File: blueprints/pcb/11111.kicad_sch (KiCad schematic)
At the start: 64 parts, among them J1 AudioJack4, SW1 SW_Push, SW10 SW_Push, SW11 SW_Push, SW12 SW_Push, SW13 SW_Push, SW14 SW_Push, SW15 SW_Push, SW16 SW_Push, SW17 SW_Push, SW18 SW_Push, SW19 SW_Push, SW2 SW_Push, SW20 SW_Push, SW21 SW_Push, SW22 SW_Push, SW23 SW_Push, SW24 SW_Push, SW25 SW_Push, SW26 SW_Push, SW27 SW_Push, SW28 SW_Push, SW29 SW_Push, SW3 SW_Push, SW30 SW_Push, SW31 SW_Push, SW4 SW_Push, SW5 SW_Push, SW6 SW_Push, SW7 SW_Push, SW8 SW_Push, SW9 SW_Push

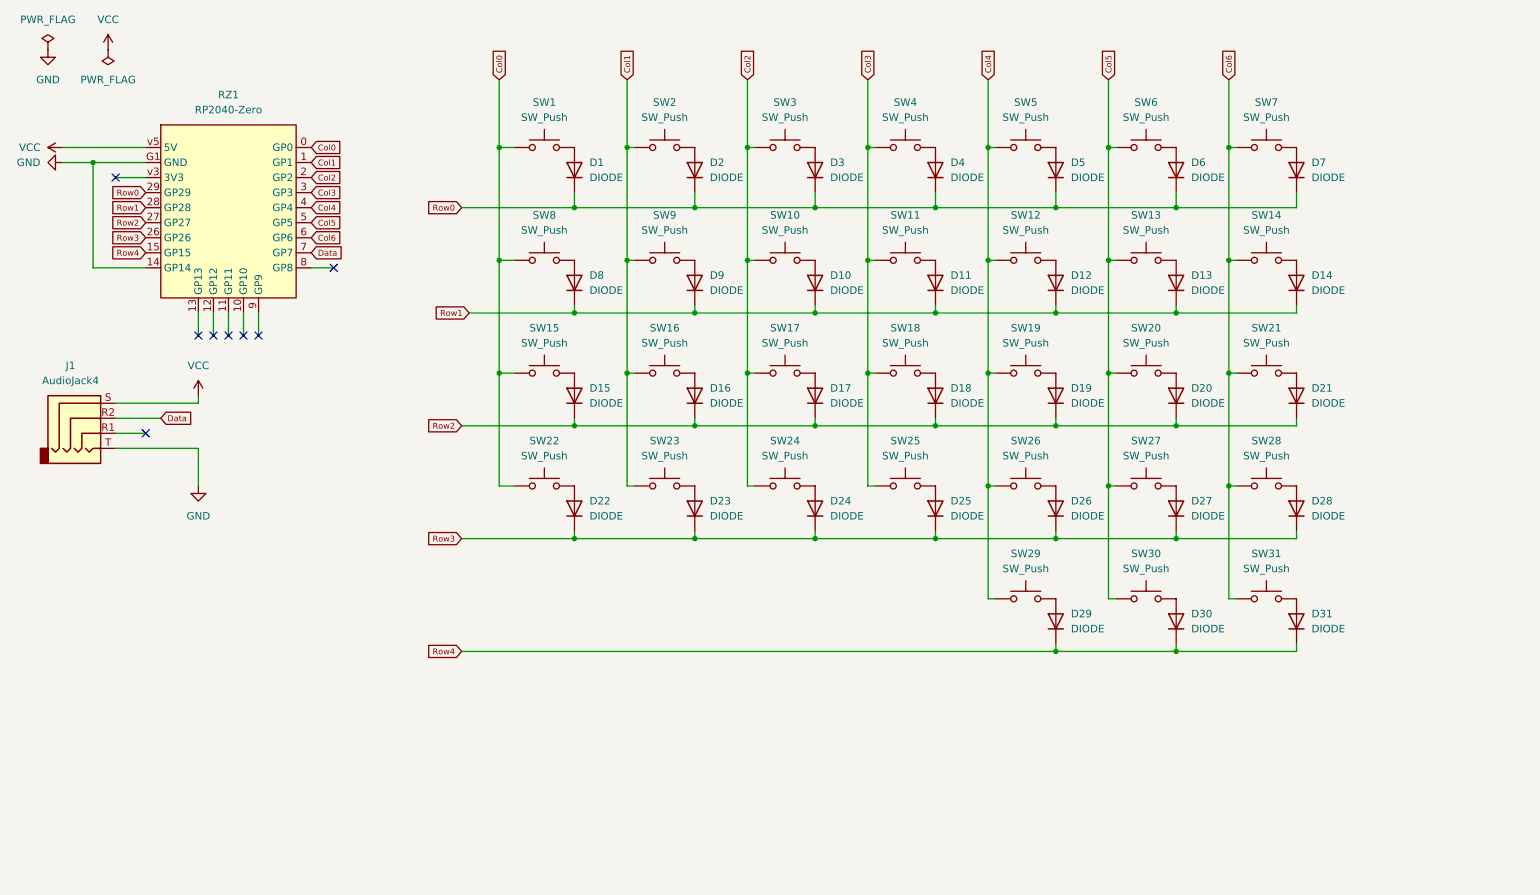
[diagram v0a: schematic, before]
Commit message: add right schematic
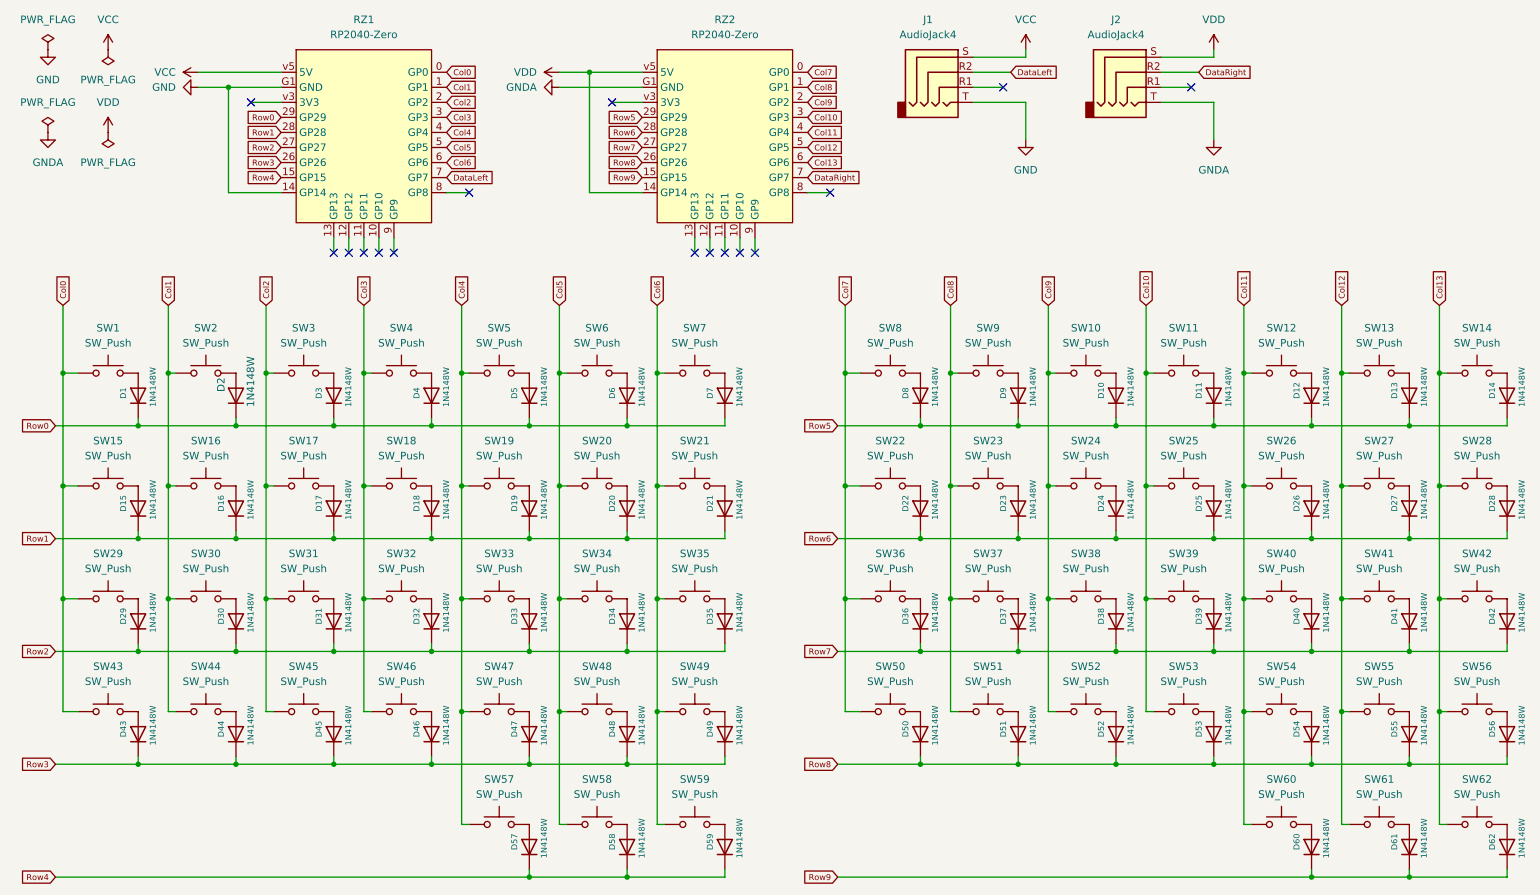
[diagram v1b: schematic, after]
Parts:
- removed D1, D10, D11, D12, D13, D14, D15, D16, D17, D18, D19, D2, D20, D21, D22, D23, D24, D25, D26, D27, D28, D29, D3, D30, D31, D4, D5, D6, D7, D8, D9: DIODE, symbol Simulation_SPICE:DIODE
- added D1, D10, D11, D12, D13, D14, D15, D16, D17, D18, D19, D2, D20, D21, D22, D23, D24, D25, D26, D27, D28, D29, D3, D30, D31, D32, D33, D34, D35, D36, D37, D38, D39, D4, D40, D41, D42, D43, D44, D45, D46, D47, D48, D49, D5, D50, D51, D52, D53, D54, D55, D56, D57, D58, D59, D6, D60, D61, D62, D7, D8, D9: 1N4148W, Diode_SMD:D_SOD-123, symbol Diode:1N4148W
- added J2: AudioJack4, symbol Connector:AudioJack4
- added RZ2: RP2040-Zero, symbol keyboard_utils:RP2040-Zero
- added SW10, SW11, SW12, SW13, SW14, SW22, SW23, SW24, SW25, SW26, SW27, SW28, SW36, SW37, SW38, SW39, SW40, SW41, SW42, SW50, SW51, SW52, SW53, SW54, SW55, SW56, SW60, SW61, SW62, SW8, SW9: SW_Push, symbol Switch:SW_Push
- renumbered SW8 to SW15, SW9 to SW16, SW10 to SW17, SW11 to SW18, SW12 to SW19, SW13 to SW20, SW14 to SW21, SW15 to SW29, SW16 to SW30, SW17 to SW31, SW18 to SW32, SW19 to SW33, SW20 to SW34, SW21 to SW35, SW22 to SW43, SW23 to SW44, SW24 to SW45, SW25 to SW46, SW26 to SW47, SW27 to SW48, SW28 to SW49, SW29 to SW57, SW30 to SW58, SW31 to SW59
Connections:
- net Row0: now also D1.1 (K), D2.1 (K), D3.1 (K), D4.1 (K), D5.1 (K), D6.1 (K), D7.1 (K)
- net Row1: now also D15.1 (K), D16.1 (K), D17.1 (K), D18.1 (K), D19.1 (K), D20.1 (K), D21.1 (K)
- net Row2: now also D29.1 (K), D30.1 (K), D31.1 (K), D32.1 (K), D33.1 (K), D34.1 (K), D35.1 (K)
- net Row3: now also D43.1 (K), D44.1 (K), D45.1 (K), D46.1 (K), D47.1 (K), D48.1 (K), D49.1 (K)
- net Row4: now also D57.1 (K), D58.1 (K), D59.1 (K)
- net at SW32.2: now also D32.2 (A)
- net at SW16.2: now also D16.2 (A)
- net at SW57.2: now also D57.2 (A)
- net at SW3.2: now also D3.2 (A)
- net at SW7.2: now also D7.2 (A)
- net at SW31.2: now also D31.2 (A)
- net at SW20.2: now also D20.2 (A)
- net at SW29.2: now also D29.2 (A)
- net at SW49.2: now also D49.2 (A)
- net at SW6.2: now also D6.2 (A)
- net at SW34.2: now also D34.2 (A)
- net at SW45.2: now also D45.2 (A)
- net at SW1.2: now also D1.2 (A)
- net at SW33.2: now also D33.2 (A)
- net at SW15.2: now also D15.2 (A)
- net at SW43.2: now also D43.2 (A)
- net at SW35.2: now also D35.2 (A)
- net at SW47.2: now also D47.2 (A)
- net at SW59.2: now also D59.2 (A)
- net at SW21.2: now also D21.2 (A)
- net at SW17.2: now also D17.2 (A)
- net at SW46.2: now also D46.2 (A)
- net at SW18.2: now also D18.2 (A)
- net at SW44.2: now also D44.2 (A)
- net at SW48.2: now also D48.2 (A)
- net at SW5.2: now also D5.2 (A)
- net at SW4.2: now also D4.2 (A)
- net at SW2.2: now also D2.2 (A)
- net at SW58.2: now also D58.2 (A)
- net at SW30.2: now also D30.2 (A)
- net at SW19.2: now also D19.2 (A)
- net Data renamed DataLeft
- new net: D13.2 (A), SW13.2
- new net: D25.2 (A), SW25.2
- new net: D56.2 (A), SW56.2
- new net: D40.2 (A), SW40.2
- new net: D23.2 (A), SW23.2
- new net: D14.2 (A), SW14.2
- new net: D28.2 (A), SW28.2
- new net: D55.2 (A), SW55.2
- new net: D37.2 (A), SW37.2
- new net: D50.2 (A), SW50.2
- new net: D42.2 (A), SW42.2
- new net: D52.2 (A), SW52.2
- new net: D22.2 (A), SW22.2
- new net: D54.2 (A), SW54.2
- new net: D26.2 (A), SW26.2
- new net: D8.2 (A), SW8.2
- new net: D62.2 (A), SW62.2
- new net: D41.2 (A), SW41.2
- new net: D61.2 (A), SW61.2
- new net: D38.2 (A), SW38.2
- new net: D10.2 (A), SW10.2
- new net: D39.2 (A), SW39.2
- new net: D24.2 (A), SW24.2
- new net: D9.2 (A), SW9.2
- new net: D60.2 (A), SW60.2
- new net: D27.2 (A), SW27.2
- new net: D11.2 (A), SW11.2
- new net: D51.2 (A), SW51.2
- new net: D12.2 (A), SW12.2
- new net: D53.2 (A), SW53.2
- new net: D36.2 (A), SW36.2
- new net Col10: RZ2.3 (GP3), SW11.1, SW25.1, SW39.1, SW53.1
- new net Col11: RZ2.4 (GP4), SW12.1, SW26.1, SW40.1, SW54.1, SW60.1
- new net Col12: RZ2.5 (GP5), SW13.1, SW27.1, SW41.1, SW55.1, SW61.1
- new net Col13: RZ2.6 (GP6), SW14.1, SW28.1, SW42.1, SW56.1, SW62.1
- new net Col7: RZ2.0 (GP0), SW22.1, SW36.1, SW50.1, SW8.1
- new net Col8: RZ2.1 (GP1), SW23.1, SW37.1, SW51.1, SW9.1
- new net Col9: RZ2.2 (GP2), SW10.1, SW24.1, SW38.1, SW52.1
- new net DataRight: J2.R2, RZ2.7 (GP7)
- new net GNDA: J2.T, RZ2.G1 (GND)
- new net Row5: D10.1 (K), D11.1 (K), D12.1 (K), D13.1 (K), D14.1 (K), D8.1 (K), D9.1 (K), RZ2.29 (GP29)
- new net Row6: D22.1 (K), D23.1 (K), D24.1 (K), D25.1 (K), D26.1 (K), D27.1 (K), D28.1 (K), RZ2.28 (GP28)
- new net Row7: D36.1 (K), D37.1 (K), D38.1 (K), D39.1 (K), D40.1 (K), D41.1 (K), D42.1 (K), RZ2.27 (GP27)
- new net Row8: D50.1 (K), D51.1 (K), D52.1 (K), D53.1 (K), D54.1 (K), D55.1 (K), D56.1 (K), RZ2.26 (GP26)
- new net Row9: D60.1 (K), D61.1 (K), D62.1 (K), RZ2.15 (GP15)
- new net VDD: J2.S, RZ2.14 (GP14), RZ2.v5 (5V)
- no-connect marks 8 -> 16
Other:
- moved on the sheet: J1, RZ1, SW1, SW15, SW16, SW17, SW18, SW19, SW2, SW20, SW21, SW29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
